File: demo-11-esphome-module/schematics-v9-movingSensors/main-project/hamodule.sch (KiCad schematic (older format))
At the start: 55 parts, among them J1 1017505, J2 Conn-ESP-Relays, J3 1017505, J4 Conn-Buttons, J5 Conn_01x02, J6 Conn-Esp-Sensors, J7 Conn-LedIndicators, J8 1017505, K1 G5Q-1, K2 G5Q-1, K3 G5Q-1, K4 G5Q-1, U1 ULN2003A, U2 LD1117S33TR_SOT223, U3 HCPL3700, U4 HCPL3700, U5 HCPL3700, U6 HCPL3700

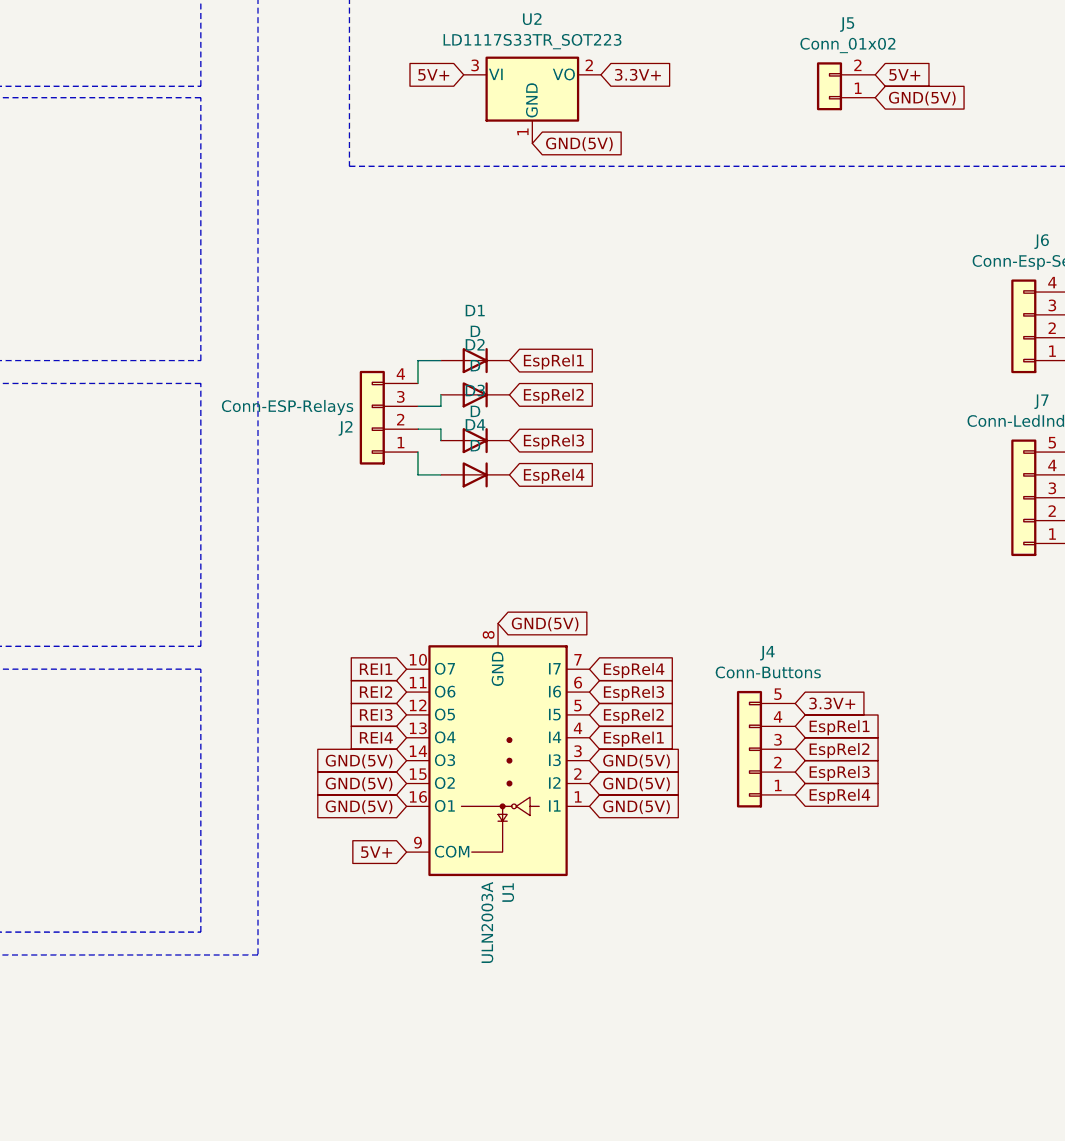
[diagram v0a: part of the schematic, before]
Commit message: can't remember
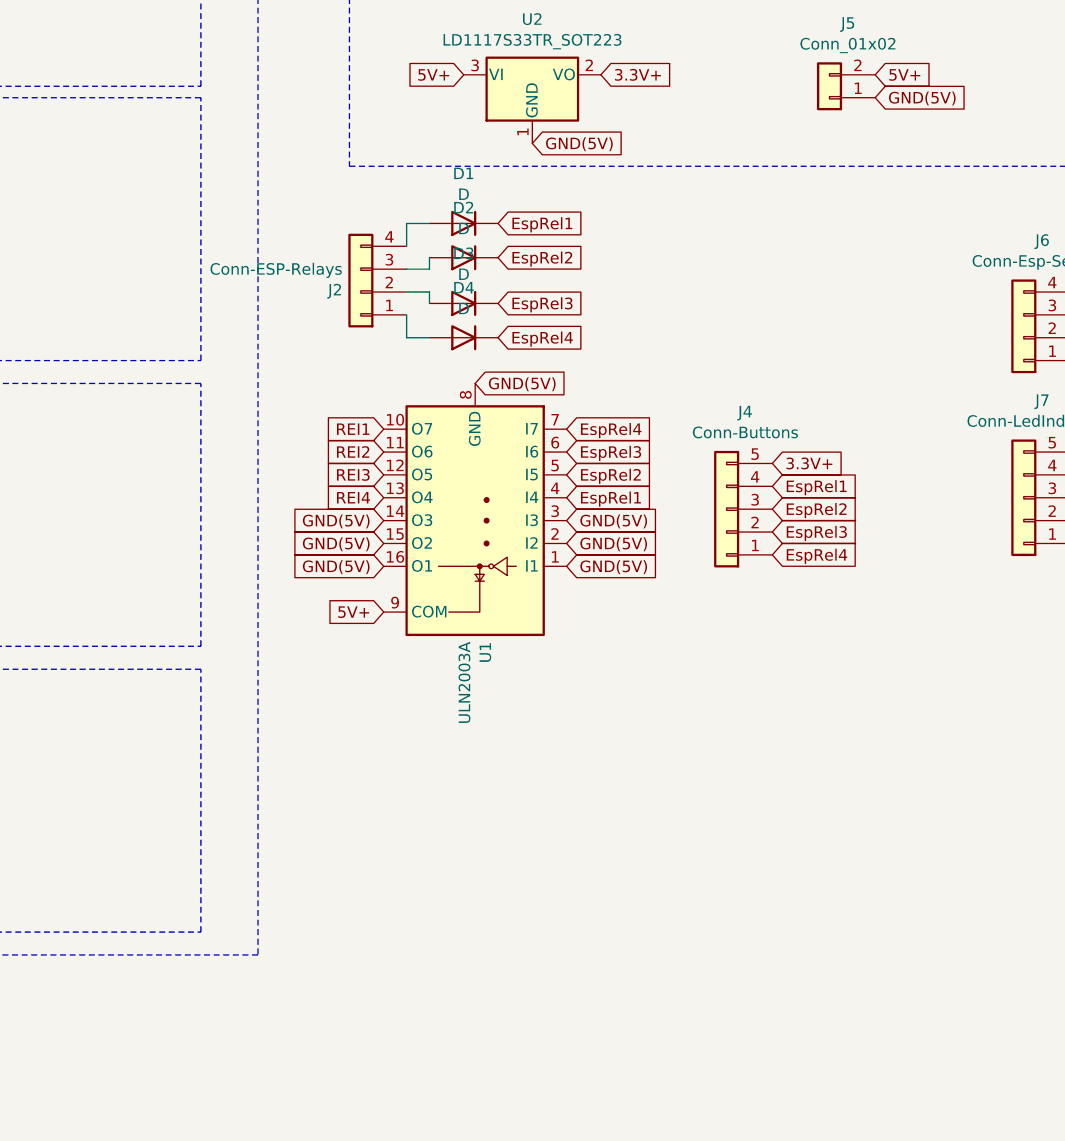
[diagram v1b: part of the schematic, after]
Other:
- moved on the sheet: D1, D2, D3, D4, J2, J4, U1
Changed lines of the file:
@@
 Wire Wire Line
 	4100 1600 4100 1900
-Text GLabel 4450 5050 2    50   Input ~ 0
-GND(5V)
-Text GLabel 4850 5750 2    50   Input ~ 0
-GND(5V)
-Text GLabel 4850 5650 2    50   Input ~ 0
-GND(5V)
-Text GLabel 4850 5850 2    50   Input ~ 0
-GND(5V)
-Text GLabel 4050 5850 0    50   Input ~ 0
-GND(5V)
-Text GLabel 4050 5750 0    50   Input ~ 0
-GND(5V)
-Text GLabel 4050 5650 0    50   Input ~ 0
-GND(5V)
-Text GLabel 4050 5550 0    50   Input ~ 0
+Text GLabel 4350 4000 2    50   Input ~ 0
+GND(5V)
+Text GLabel 4750 4700 2    50   Input ~ 0
+GND(5V)
+Text GLabel 4750 4600 2    50   Input ~ 0
+GND(5V)
+Text GLabel 4750 4800 2    50   Input ~ 0
+GND(5V)
+Text GLabel 3950 4800 0    50   Input ~ 0
+GND(5V)
+Text GLabel 3950 4700 0    50   Input ~ 0
+GND(5V)
+Text GLabel 3950 4600 0    50   Input ~ 0
+GND(5V)
+Text GLabel 3950 4500 0    50   Input ~ 0
 REI4
-Text GLabel 4050 5450 0    50   Input ~ 0
+Text GLabel 3950 4400 0    50   Input ~ 0
 REI3
-Text GLabel 4050 5350 0    50   Input ~ 0
+Text GLabel 3950 4300 0    50   Input ~ 0
 REI2
-Text GLabel 4050 5250 0    50   Input ~ 0
+Text GLabel 3950 4200 0    50   Input ~ 0
 REI1
-Text GLabel 4050 6050 0    50   Input ~ 0
+Text GLabel 3950 5000 0    50   Input ~ 0
 5V+
 $Comp
 L Transistor_Array:ULN2003A U1
 U 1 1 61374AC1
-P 4450 5650
-F 0 "U1" V 4404 6180 50  0000 L CNN
-F 1 "ULN2003A" V 4495 6180 50  0000 L CNN
-F 2 "Package_DIP:DIP-16_W7.62mm_LongPads" H 4500 5100 50  0001 L CNN
-F 3 "http://www.ti.com/lit/ds/symlink/uln2003a.pdf" H 4550 5450 50  0001 C CNN
-	1    4450 5650
+P 4350 4600
+F 0 "U1" V 4304 5130 50  0000 L CNN
+F 1 "ULN2003A" V 4395 5130 50  0000 L CNN
+F 2 "Package_DIP:DIP-16_W7.62mm_LongPads" H 4400 4050 50  0001 L CNN
+F 3 "http://www.ti.com/lit/ds/symlink/uln2003a.pdf" H 4450 4400 50  0001 C CNN
+	1    4350 4600
 	-1   0    0    1
 $EndComp
@@
 L Connector_Generic:Conn_01x05 J4
 U 1 1 61516260
-P 5550 5600
-F 0 "J4" H 5468 5175 50  0000 C CNN
-F 1 "Conn-Buttons" H 5468 5266 50  0000 C CNN
-F 2 "Connector_JST:JST_XH_B5B-XH-A_1x05_P2.50mm_Vertical" H 5550 5600 50  0001 C CNN
-F 3 "~" H 5550 5600 50  0001 C CNN
-	1    5550 5600
-	-1   0    0    1
-$EndComp
-Text GLabel 5750 5500 2    50   Input ~ 0
+P 5450 4550
+F 0 "J4" H 5368 4125 50  0000 C CNN
+F 1 "Conn-Buttons" H 5368 4216 50  0000 C CNN
+F 2 "Connector_JST:JST_XH_B5B-XH-A_1x05_P2.50mm_Vertical" H 5450 4550 50  0001 C CNN
+F 3 "~" H 5450 4550 50  0001 C CNN
+	1    5450 4550
+	-1   0    0    1
+$EndComp
+Text GLabel 5650 4450 2    50   Input ~ 0
 EspRel1
-Text GLabel 5750 5600 2    50   Input ~ 0
+Text GLabel 5650 4550 2    50   Input ~ 0
 EspRel2
-Text GLabel 5750 5700 2    50   Input ~ 0
+Text GLabel 5650 4650 2    50   Input ~ 0
 EspRel3
-Text GLabel 5750 5800 2    50   Input ~ 0
+Text GLabel 5650 4750 2    50   Input ~ 0
 EspRel4
 Text GLabel 8200 4500 0    50   Input ~ 0
@@
 Text GLabel 1100 2400 0    50   Input ~ 0
 5V+
-Text GLabel 4500 3900 2    50   Input ~ 0
+Text GLabel 4450 3300 2    50   Input ~ 0
 EspRel1
-Text GLabel 4500 4050 2    50   Input ~ 0
+Text GLabel 4450 3450 2    50   Input ~ 0
 EspRel2
-Text GLabel 4500 4250 2    50   Input ~ 0
+Text GLabel 4450 3650 2    50   Input ~ 0
 EspRel3
-Text GLabel 4500 4400 2    50   Input ~ 0
+Text GLabel 4450 3800 2    50   Input ~ 0
 EspRel4
-Text GLabel 4850 5550 2    50   Input ~ 0
+Text GLabel 4750 4500 2    50   Input ~ 0
 EspRel1
-Text GLabel 4850 5450 2    50   Input ~ 0
+Text GLabel 4750 4400 2    50   Input ~ 0
 EspRel2
-Text GLabel 4850 5350 2    50   Input ~ 0
+Text GLabel 4750 4300 2    50   Input ~ 0
 EspRel3
-Text GLabel 4850 5250 2    50   Input ~ 0
+Text GLabel 4750 4200 2    50   Input ~ 0
 EspRel4
-Text GLabel 5750 5400 2    50   Input ~ 0
-3.3V+
-Wire Wire Line
-	4200 4100 4100 4100
-Wire Wire Line
-	4100 4200 4200 4200
+Text GLabel 5650 4350 2    50   Input ~ 0
+3.3V+
+Wire Wire Line
+	4150 3500 4050 3500
+Wire Wire Line
+	4050 3600 4150 3600
 Text GLabel 9600 1650 0    50   Input ~ 0
 Sens4
@@
 L Connector_Generic:Conn_01x04 J2
 U 1 1 614144AF
-P 3900 4200
-F 0 "J2" H 3980 4192 50  0000 L CNN
-F 1 "Conn-ESP-Relays" H 3980 4101 50  0000 L CNN
-F 2 "Connector_JST:JST_XH_B4B-XH-A_1x04_P2.50mm_Vertical" H 3900 4200 50  0001 C CNN
-F 3 "~" H 3900 4200 50  0001 C CNN
-	1    3900 4200
+P 3850 3600
+F 0 "J2" H 3930 3592 50  0000 L CNN
+F 1 "Conn-ESP-Relays" H 3930 3501 50  0000 L CNN
+F 2 "Connector_JST:JST_XH_B4B-XH-A_1x04_P2.50mm_Vertical" H 3850 3600 50  0001 C CNN
+F 3 "~" H 3850 3600 50  0001 C CNN
+	1    3850 3600
 	-1   0    0    1
 $EndComp
@@
 L Device:D D1
 U 1 1 615714B6
-P 4350 3900
-F 0 "D1" H 4350 3683 50  0000 C CNN
-F 1 "D" H 4350 3774 50  0000 C CNN
-F 2 "Diode_THT:D_A-405_P7.62mm_Horizontal" H 4350 3900 50  0001 C CNN
-F 3 "~" H 4350 3900 50  0001 C CNN
-	1    4350 3900
+P 4300 3300
+F 0 "D1" H 4300 3083 50  0000 C CNN
+F 1 "D" H 4300 3174 50  0000 C CNN
+F 2 "Diode_THT:D_A-405_P7.62mm_Horizontal" H 4300 3300 50  0001 C CNN
+F 3 "~" H 4300 3300 50  0001 C CNN
+	1    4300 3300
 	-1   0    0    1
 $EndComp
@@
 L Device:D D2
 U 1 1 615764D6
-P 4350 4050
-F 0 "D2" H 4350 3833 50  0000 C CNN
-F 1 "D" H 4350 3924 50  0000 C CNN
-F 2 "Diode_THT:D_A-405_P7.62mm_Horizontal" H 4350 4050 50  0001 C CNN
-F 3 "~" H 4350 4050 50  0001 C CNN
-	1    4350 4050
+P 4300 3450
+F 0 "D2" H 4300 3233 50  0000 C CNN
+F 1 "D" H 4300 3324 50  0000 C CNN
+F 2 "Diode_THT:D_A-405_P7.62mm_Horizontal" H 4300 3450 50  0001 C CNN
+F 3 "~" H 4300 3450 50  0001 C CNN
+	1    4300 3450
 	-1   0    0    1
 $EndComp
@@
 L Device:D D3
 U 1 1 615780DE
-P 4350 4250
-F 0 "D3" H 4350 4033 50  0000 C CNN
-F 1 "D" H 4350 4124 50  0000 C CNN
-F 2 "Diode_THT:D_A-405_P7.62mm_Horizontal" H 4350 4250 50  0001 C CNN
-F 3 "~" H 4350 4250 50  0001 C CNN
-	1    4350 4250
+P 4300 3650
+F 0 "D3" H 4300 3433 50  0000 C CNN
+F 1 "D" H 4300 3524 50  0000 C CNN
+F 2 "Diode_THT:D_A-405_P7.62mm_Horizontal" H 4300 3650 50  0001 C CNN
+F 3 "~" H 4300 3650 50  0001 C CNN
+	1    4300 3650
 	-1   0    0    1
 $EndComp
@@
 L Device:D D4
 U 1 1 6157A0C6
-P 4350 4400
-F 0 "D4" H 4350 4183 50  0000 C CNN
-F 1 "D" H 4350 4274 50  0000 C CNN
-F 2 "Diode_THT:D_A-405_P7.62mm_Horizontal" H 4350 4400 50  0001 C CNN
-F 3 "~" H 4350 4400 50  0001 C CNN
-	1    4350 4400
-	-1   0    0    1
-$EndComp
-Wire Wire Line
-	4200 3900 4100 3900
-Wire Wire Line
-	4100 3900 4100 4000
-Wire Wire Line
-	4200 4400 4100 4400
-Wire Wire Line
-	4100 4400 4100 4300
-Wire Wire Line
-	4200 4250 4200 4200
-Wire Wire Line
-	4200 4050 4200 4100
+P 4300 3800
+F 0 "D4" H 4300 3583 50  0000 C CNN
+F 1 "D" H 4300 3674 50  0000 C CNN
+F 2 "Diode_THT:D_A-405_P7.62mm_Horizontal" H 4300 3800 50  0001 C CNN
+F 3 "~" H 4300 3800 50  0001 C CNN
+	1    4300 3800
+	-1   0    0    1
+$EndComp
+Wire Wire Line
+	4150 3300 4050 3300
+Wire Wire Line
+	4050 3300 4050 3400
+Wire Wire Line
+	4150 3800 4050 3800
+Wire Wire Line
+	4050 3800 4050 3700
+Wire Wire Line
+	4150 3650 4150 3600
+Wire Wire Line
+	4150 3450 4150 3500
 $EndSCHEMATC
